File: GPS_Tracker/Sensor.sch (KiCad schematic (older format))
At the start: 3 parts

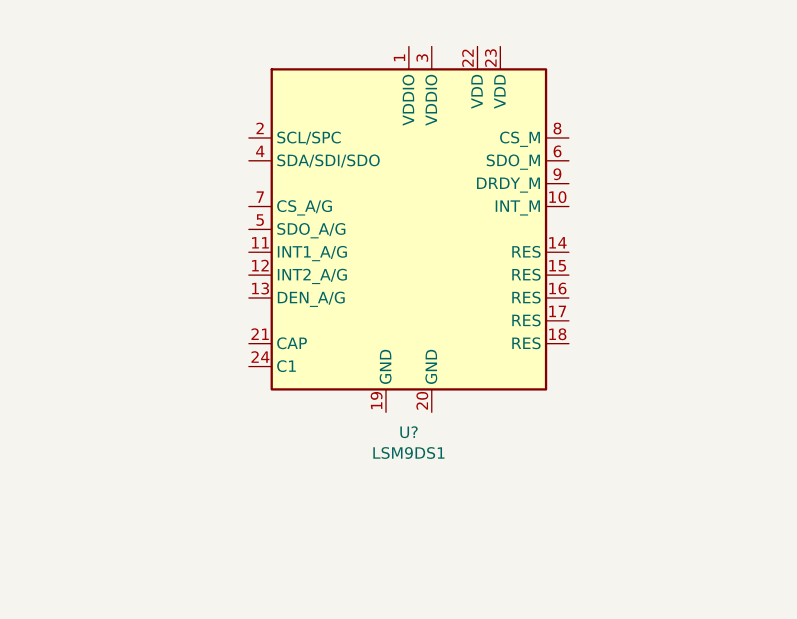
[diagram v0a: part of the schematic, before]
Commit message: started 9dof
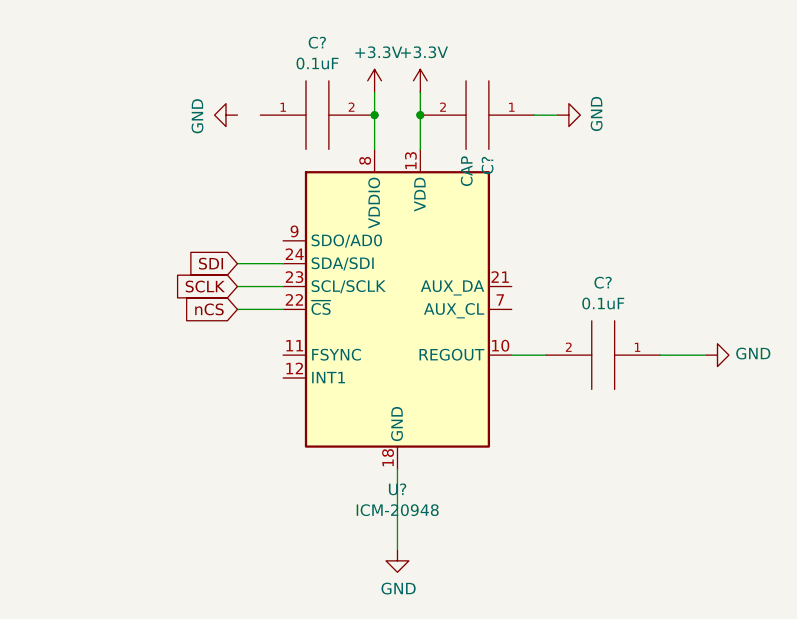
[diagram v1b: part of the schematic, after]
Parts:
- removed U?: LSM9DS1, Package_LGA:LGA-24L_3x3.5mm_P0.43mm, symbol Sensor_Motion:LSM9DS1
- added C? (x2): 0.1uF, symbol pspice:CAP
- added C?: CAP, symbol pspice:CAP
- added U?: ICM-20948, Sensor_Motion:InvenSense_QFN-24_3x3mm_P0.4mm, symbol Sensor_Motion:ICM-20948
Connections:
- net +3V3: now also C?.2, C?.2, U?.13 (VDD), U?.8 (VDDIO)
- net GND: now also C?.1, C?.1, U?.18 (GND), U?.20 (GND)
- new net: C?.2, U?.10 (REGOUT)
- new net SCLK: U?.23 (SCL/SCLK)
- new net SDI: U?.24 (SDA/SDI)
- new net nCS: U?.22 (~CS)
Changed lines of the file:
@@
 $Descr A4 11693 8268
 encoding utf-8
-Sheet 1 7
+Sheet 1 1
 Title ""
 Date ""
@@
 Wire Wire Line
 	2450 2350 2450 2200
-$Comp
-L Sensor_Motion:LSM9DS1 U?
-U 1 1 5E729015
-P 7650 2900
-F 0 "U?" H 7650 2011 50  0000 C CNN
-F 1 "LSM9DS1" H 7650 1920 50  0000 C CNN
-F 2 "Package_LGA:LGA-24L_3x3.5mm_P0.43mm" H 9150 3650 50  0001 C CNN
-F 3 "http://www.st.com/content/ccc/resource/technical/document/datasheet/1e/3f/2a/d6/25/eb/48/46/DM00103319.pdf/files/DM00103319.pdf/jcr:content/translations/en.DM00103319.pdf" H 7650 3000 50  0001 C CNN
-	1    7650 2900
-	1    0    0    -1
-$EndComp
 Text HLabel 1650 3050 0    50   Input ~ 0
 SCL
 Text HLabel 1650 2950 0    50   Input ~ 0
 SDA
+$Comp
+L Sensor_Motion:ICM-20948 U?
+U 1 1 5E72C53E
+P 7600 3250
+F 0 "U?" H 7600 2461 50  0000 C CNN
+F 1 "ICM-20948" H 7600 2370 50  0000 C CNN
+F 2 "Sensor_Motion:InvenSense_QFN-24_3x3mm_P0.4mm" H 7600 2250 50  0001 C CNN
+F 3 "http://www.invensense.com/wp-content/uploads/2016/06/DS-000189-ICM-20948-v1.3.pdf" H 7600 3100 50  0001 C CNN
+	1    7600 3250
+	1    0    0    -1
+$EndComp
+$Comp
+L power:GND #PWR?
+U 1 1 5E72EA31
+P 7600 4300
+F 0 "#PWR?" H 7600 4050 50  0001 C CNN
+F 1 "GND" H 7605 4127 50  0000 C CNN
+F 2 "" H 7600 4300 50  0001 C CNN
+F 3 "" H 7600 4300 50  0001 C CNN
+	1    7600 4300
+	1    0    0    -1
+$EndComp
+Wire Wire Line
+	7600 3950 7600 4300
+Text GLabel 6900 3050 0    50   Input ~ 0
+SDI
+Text GLabel 6900 3150 0    50   Input ~ 0
+SCLK
+Text GLabel 6900 3250 0    50   Input ~ 0
+nCS
+Wire Wire Line
+	6900 3050 7100 3050
+Wire Wire Line
+	6900 3150 7100 3150
+Wire Wire Line
+	6900 3250 7100 3250
+$Comp
+L power:GND #PWR?
+U 1 1 5E7302D3
+P 8300 2400
+F 0 "#PWR?" H 8300 2150 50  0001 C CNN
+F 1 "GND" H 8305 2227 50  0000 C CNN
+F 2 "" H 8300 2400 50  0001 C CNN
+F 3 "" H 8300 2400 50  0001 C CNN
+	1    8300 2400
+	0    -1   -1   0
+$EndComp
+$Comp
+L power:GND #PWR?
+U 1 1 5E730942
+P 6900 2400
+F 0 "#PWR?" H 6900 2150 50  0001 C CNN
+F 1 "GND" H 6905 2227 50  0000 C CNN
+F 2 "" H 6900 2400 50  0001 C CNN
+F 3 "" H 6900 2400 50  0001 C CNN
+	1    6900 2400
+	0    1    1    0
+$EndComp
+$Comp
+L pspice:CAP C?
+U 1 1 5E731644
+P 7250 2400
+F 0 "C?" V 7565 2400 50  0000 C CNN
+F 1 "0.1uF" V 7474 2400 50  0000 C CNN
+F 2 "" H 7250 2400 50  0001 C CNN
+F 3 "~" H 7250 2400 50  0001 C CNN
+	1    7250 2400
+	0    -1   -1   0
+$EndComp
+$Comp
+L pspice:CAP C?
+U 1 1 5E731D9C
+P 7950 2400
+F 0 "C?" H 8128 2446 50  0000 L CNN
+F 1 "CAP" H 8128 2355 50  0000 L CNN
+F 2 "" H 7950 2400 50  0001 C CNN
+F 3 "~" H 7950 2400 50  0001 C CNN
+	1    7950 2400
+	0    1    1    0
+$EndComp
+$Comp
+L power:+3.3V #PWR?
+U 1 1 5E733708
+P 7500 2300
+F 0 "#PWR?" H 7500 2150 50  0001 C CNN
+F 1 "+3.3V" H 7515 2473 50  0000 C CNN
+F 2 "" H 7500 2300 50  0001 C CNN
+F 3 "" H 7500 2300 50  0001 C CNN
+	1    7500 2300
+	1    0    0    -1
+$EndComp
+$Comp
+L power:+3.3V #PWR?
+U 1 1 5E733BE9
+P 7700 2300
+F 0 "#PWR?" H 7700 2150 50  0001 C CNN
+F 1 "+3.3V" H 7715 2473 50  0000 C CNN
+F 2 "" H 7700 2300 50  0001 C CNN
+F 3 "" H 7700 2300 50  0001 C CNN
+	1    7700 2300
+	1    0    0    -1
+$EndComp
+Wire Wire Line
+	7500 2300 7500 2400
+Wire Wire Line
+	7700 2300 7700 2400
+Connection ~ 7500 2400
+Wire Wire Line
+	7500 2400 7500 2550
+Connection ~ 7700 2400
+Wire Wire Line
+	7700 2400 7700 2550
+Wire Wire Line
+	8200 2400 8300 2400
+$Comp
+L pspice:CAP C?
+U 1 1 5E73B2C6
+P 8500 3450
+F 0 "C?" V 8185 3450 50  0000 C CNN
+F 1 "0.1uF" V 8276 3450 50  0000 C CNN
+F 2 "" H 8500 3450 50  0001 C CNN
+F 3 "~" H 8500 3450 50  0001 C CNN
+	1    8500 3450
+	0    1    1    0
+$EndComp
+$Comp
+L power:GND #PWR?
+U 1 1 5E73BEE0
+P 8950 3450
+F 0 "#PWR?" H 8950 3200 50  0001 C CNN
+F 1 "GND" V 8955 3322 50  0000 R CNN
+F 2 "" H 8950 3450 50  0001 C CNN
+F 3 "" H 8950 3450 50  0001 C CNN
+	1    8950 3450
+	0    -1   -1   0
+$EndComp
+Wire Wire Line
+	8100 3450 8250 3450
+Wire Wire Line
+	8750 3450 8950 3450
 $EndSCHEMATC
